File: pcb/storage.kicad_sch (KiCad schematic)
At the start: 5 parts, among them J401 MICRO_SD(TFC-WPAPR-08)

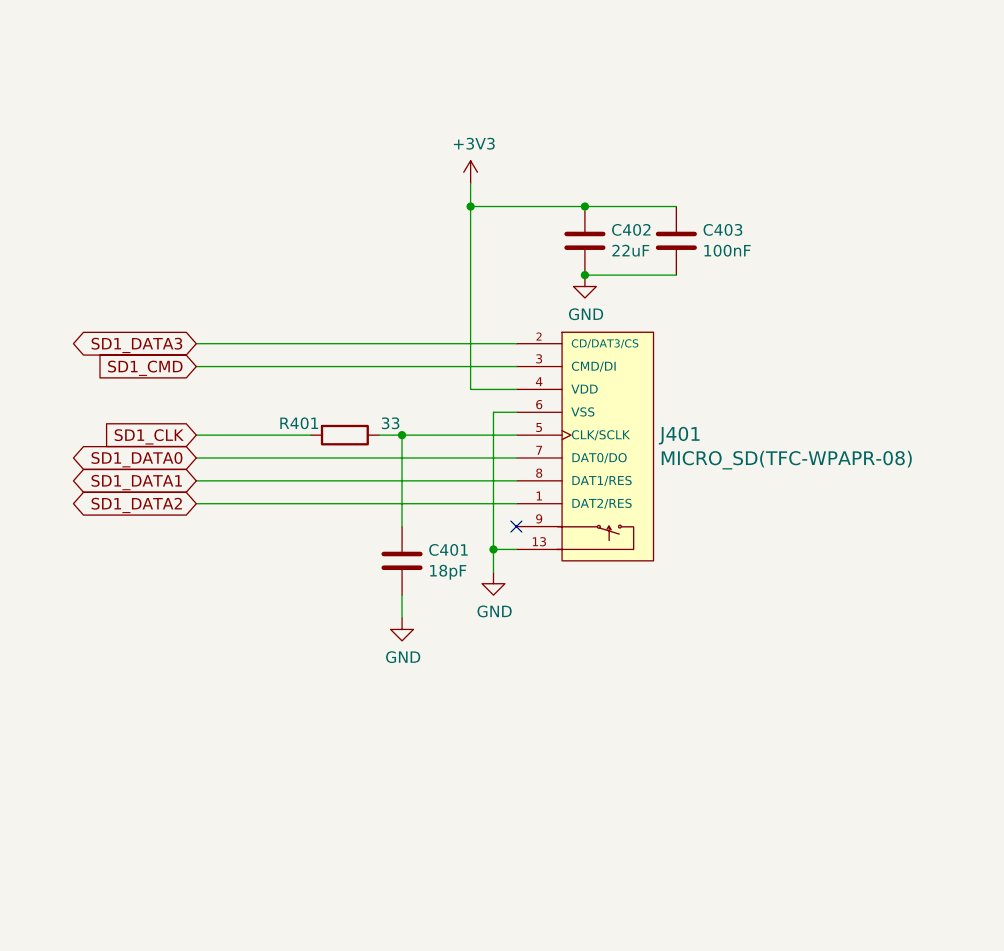
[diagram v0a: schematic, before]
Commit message: pcb: getting ready for r0.2 production
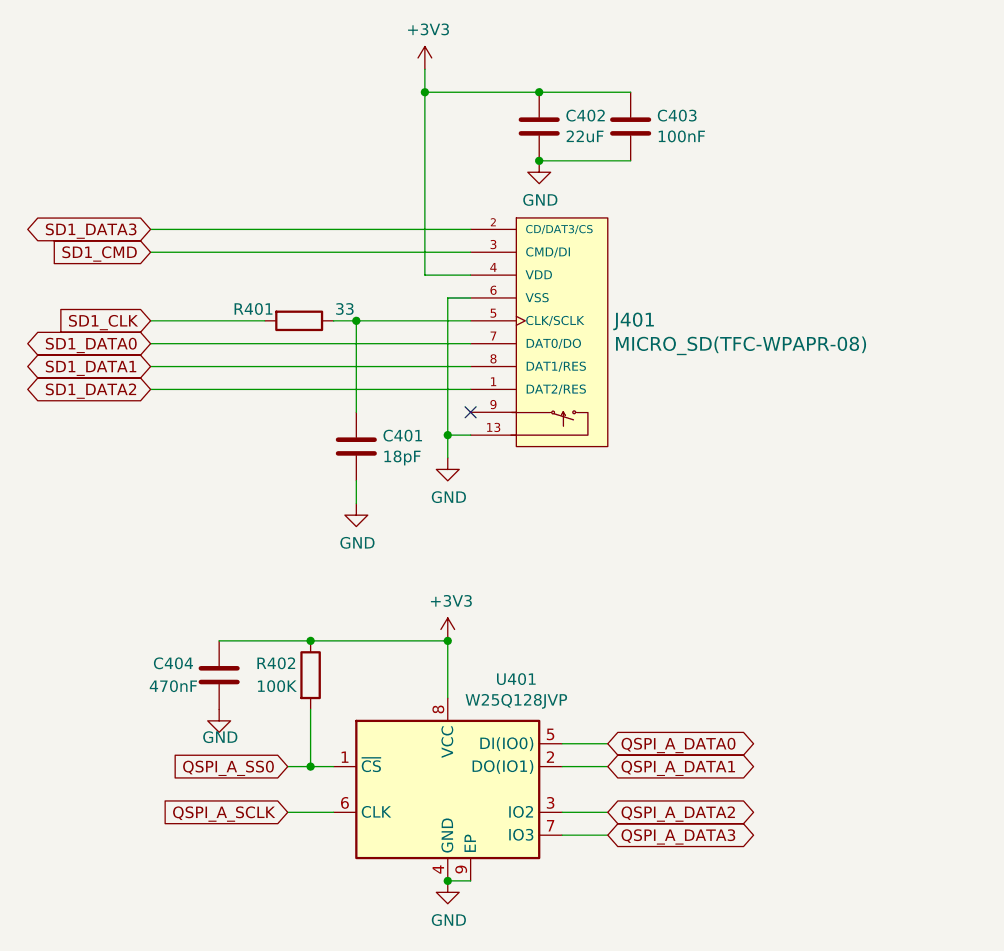
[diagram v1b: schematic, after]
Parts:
- added C404: 470nF, Capacitor_SMD:C_0402_1005Metric, symbol Device:C
- added R402: 100K, Capacitor_SMD:C_0402_1005Metric, symbol Device:R
- added U401: W25Q128JVP, Package_SON:WSON-8-1EP_6x5mm_P1.27mm_EP3.4x4.3mm, symbol Memory_Flash:W25Q32JVZP
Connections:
- net +3V3: now also C404.2, R402.1, U401.8 (VCC)
- net GND: now also C404.1, U401.4 (GND), U401.9 (EP)
- new net QSPI_A_DATA0: U401.5 (DI(IO0))
- new net QSPI_A_DATA1: U401.2 (DO(IO1))
- new net QSPI_A_DATA2: U401.3 (IO2)
- new net QSPI_A_DATA3: U401.7 (IO3)
- new net QSPI_A_SCLK: U401.6 (CLK)
- new net QSPI_A_SS0: R402.2, U401.1 (~{CS})
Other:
- moved on the sheet: C401, C402, C403, J401, R401
